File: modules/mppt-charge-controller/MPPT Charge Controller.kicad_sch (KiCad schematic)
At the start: 53 parts, among them Q1 SI7272DP, Q3 2N7002, U2 AP63203WU, U3 ACS712, U4 ACS712, U5 MCP4018

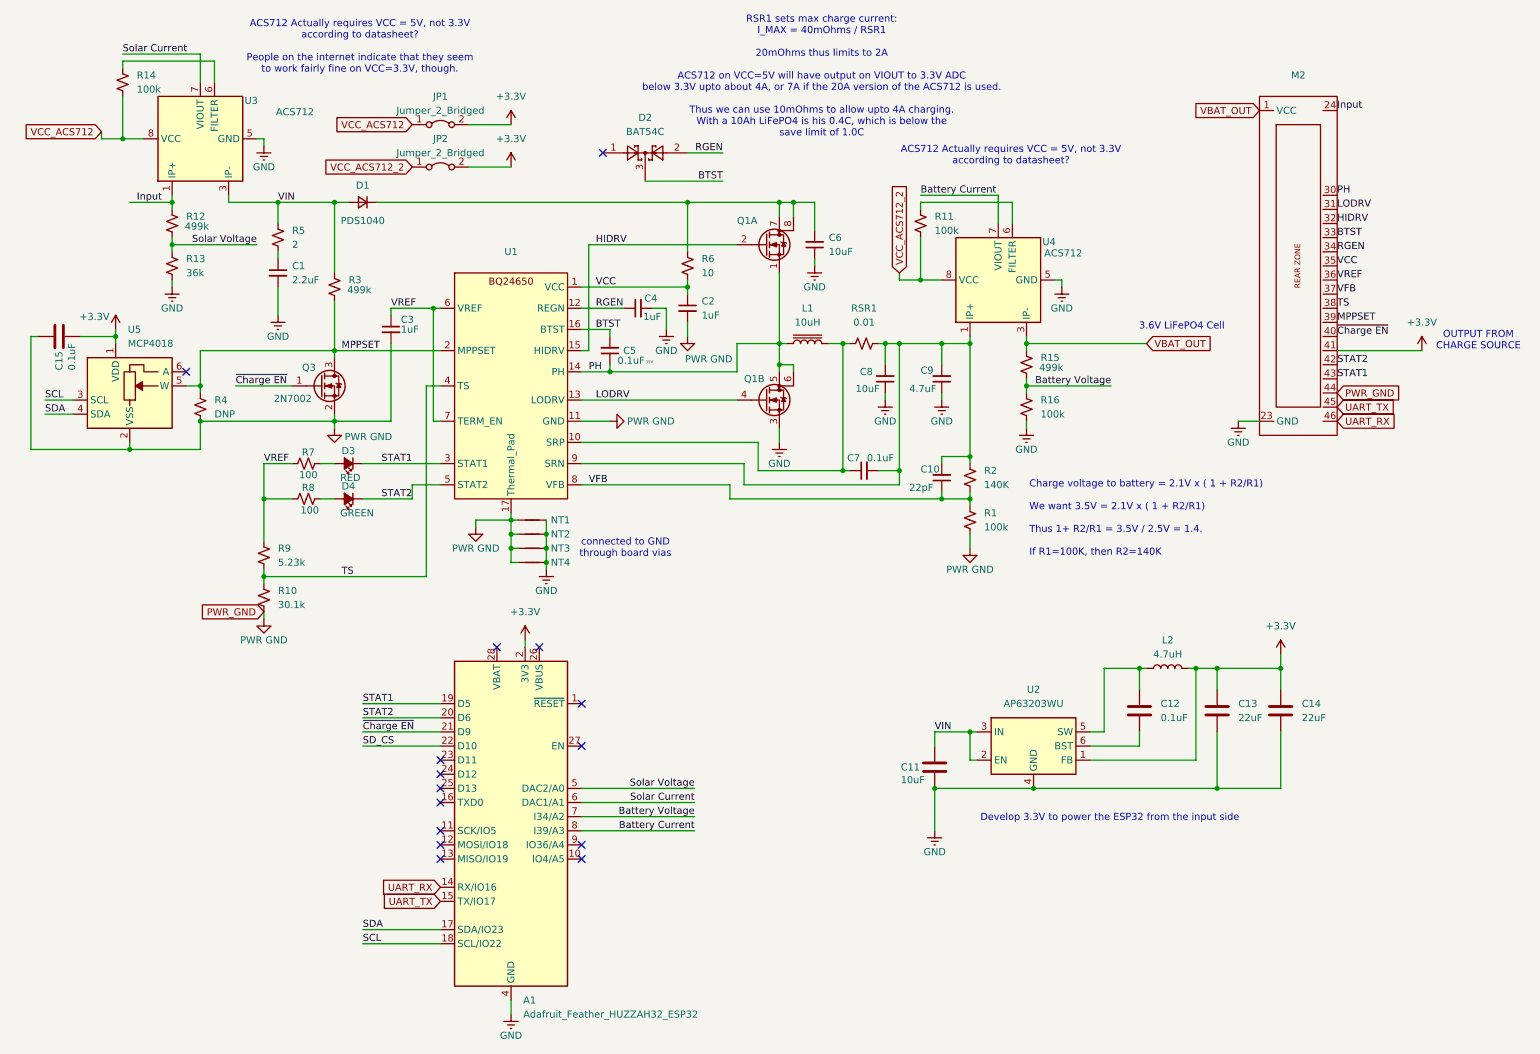
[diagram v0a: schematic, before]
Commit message: Updating all modules
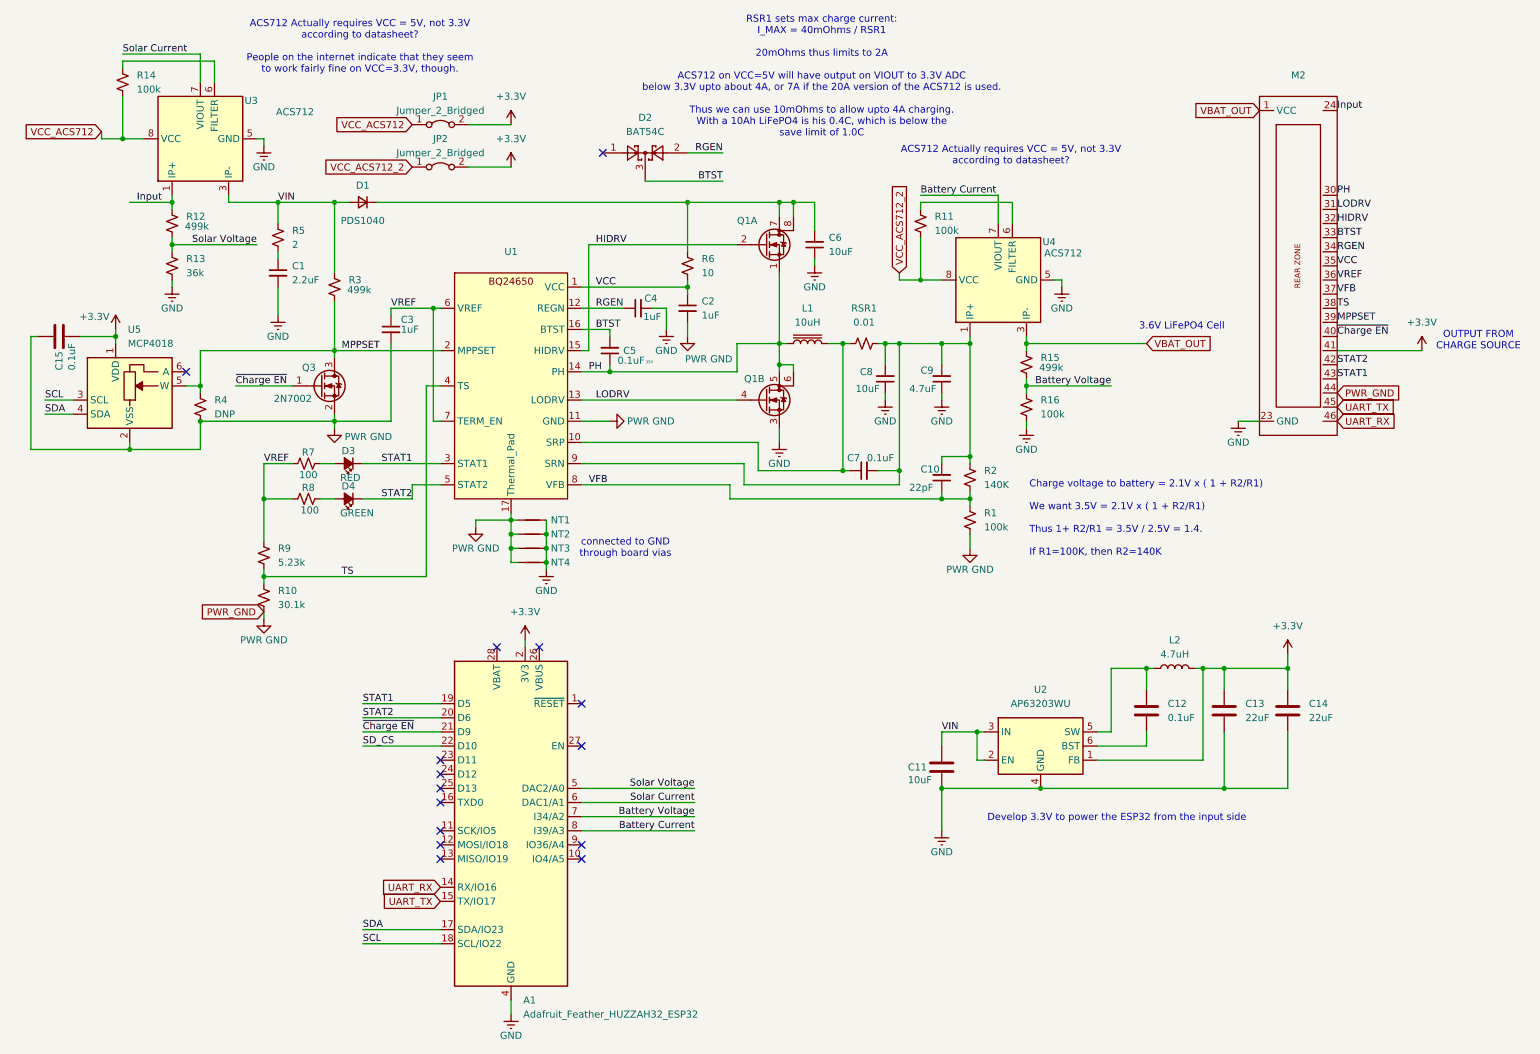
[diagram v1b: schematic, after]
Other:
- moved on the sheet: C11, C12, C13, C14, L2, U2
